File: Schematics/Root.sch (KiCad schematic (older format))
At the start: 1 part, among them CON2 BARREL_JACK

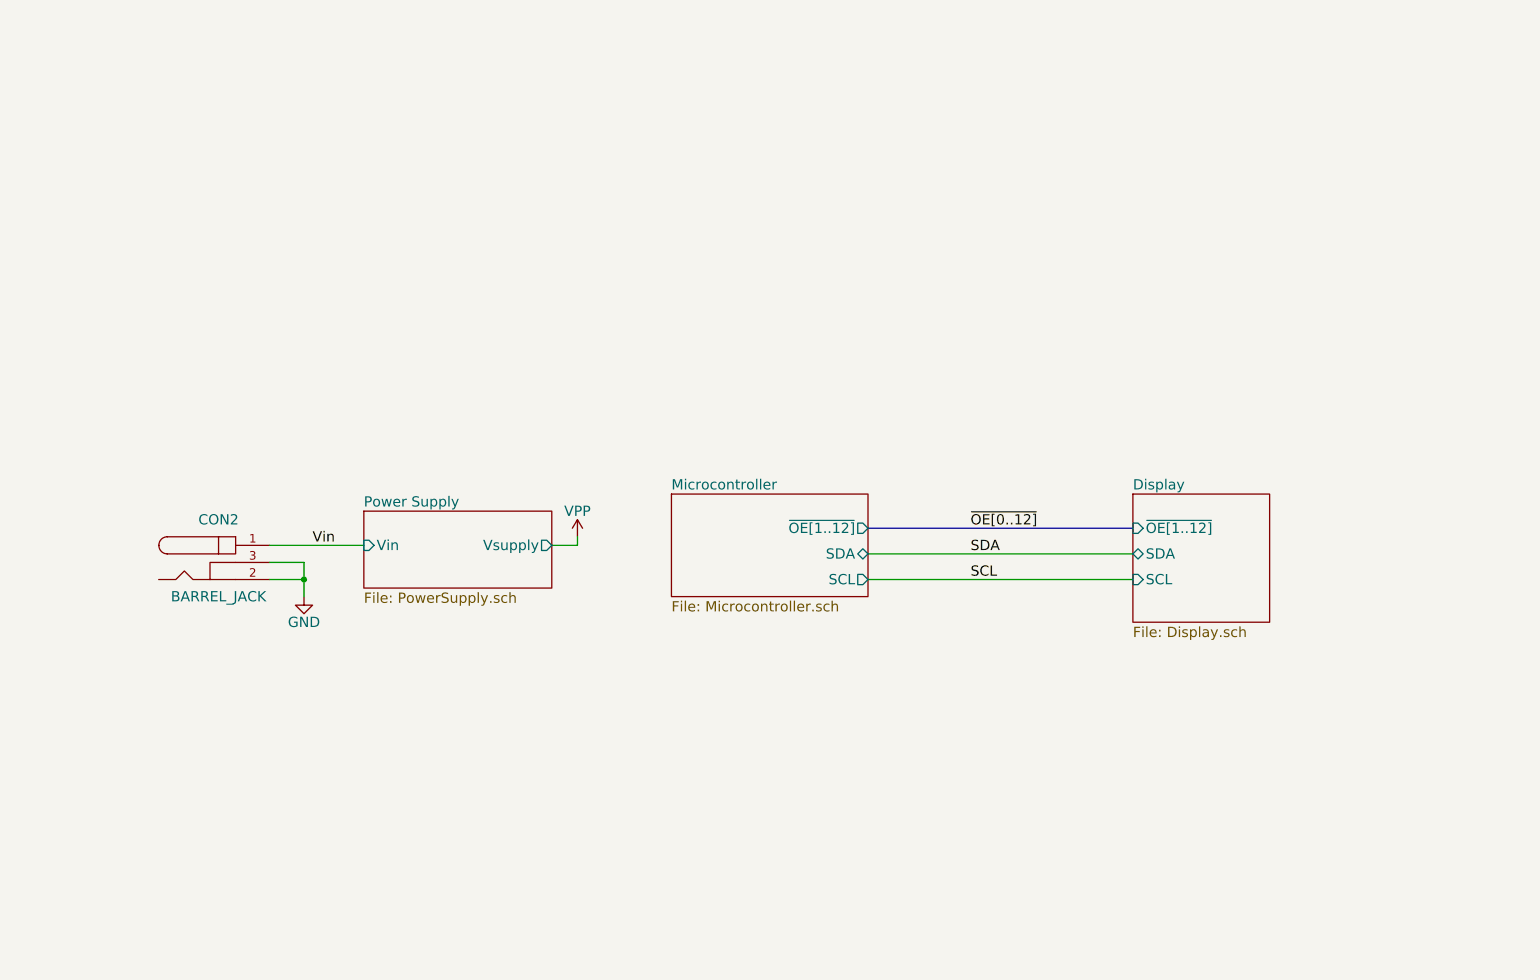
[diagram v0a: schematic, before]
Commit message: Started Redesign.
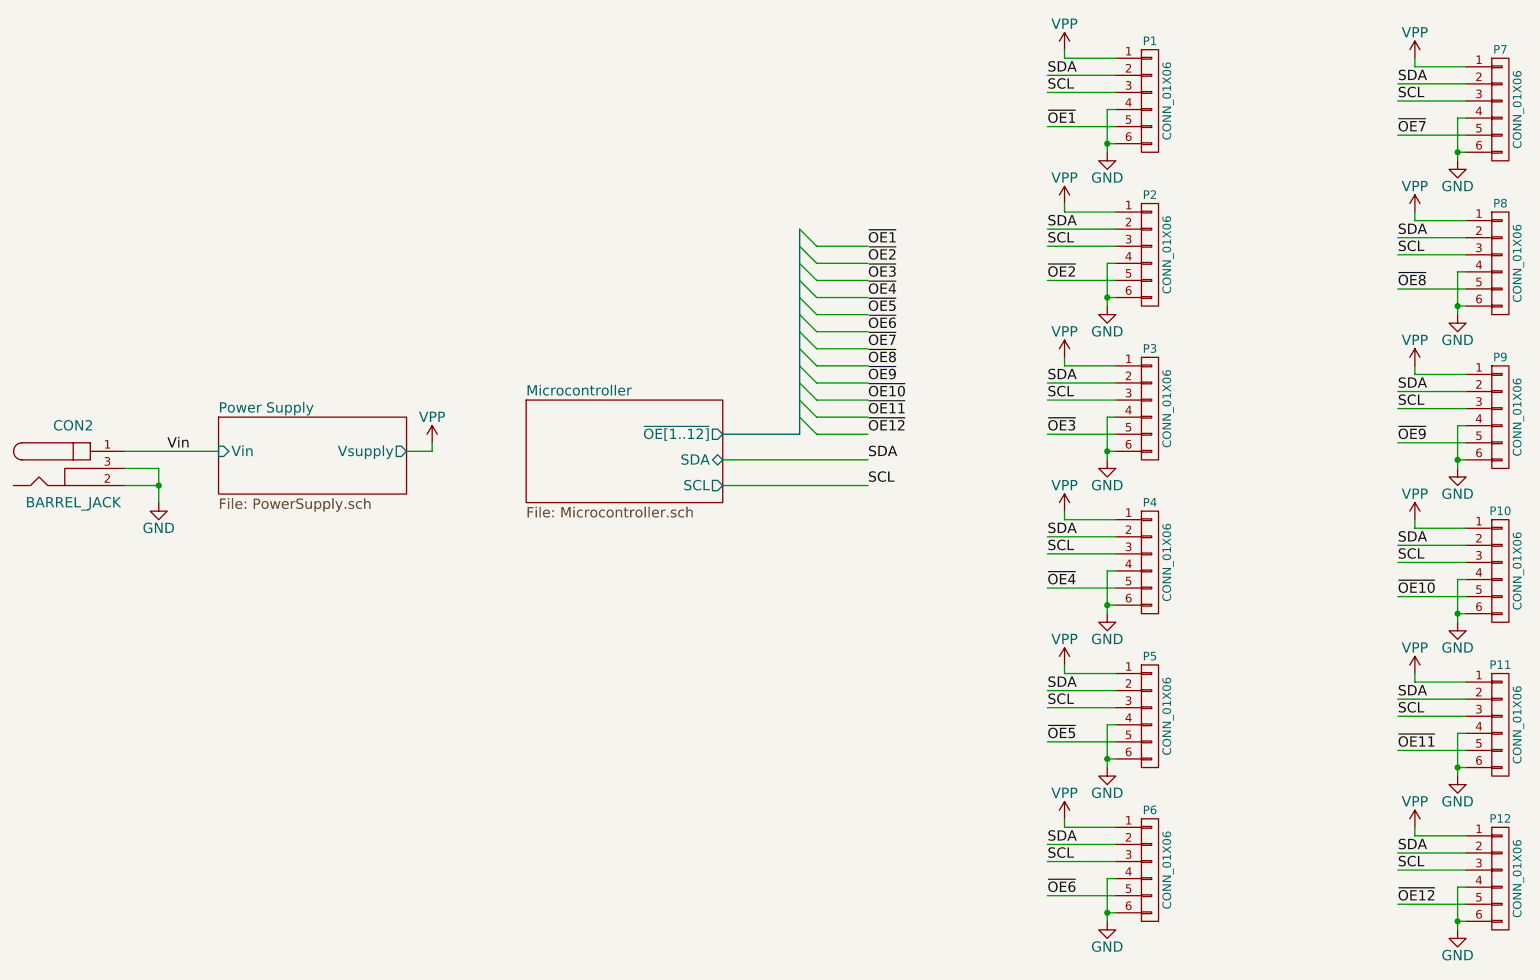
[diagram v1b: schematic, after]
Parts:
- added P1, P10, P11, P12, P2, P3, P4, P5, P6, P7, P8, P9: CONN_01X06, symbol CONN_01X06
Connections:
- net GND: now also P1.4 (P4), P1.6 (P6), P10.4 (P4), P10.6 (P6), P11.4 (P4), P11.6 (P6), P12.4 (P4), P12.6 (P6), P2.4 (P4), P2.6 (P6), P3.4 (P4), P3.6 (P6), P4.4 (P4), P4.6 (P6), P5.4 (P4), P5.6 (P6), P6.4 (P4), P6.6 (P6), P7.4 (P4), P7.6 (P6), P8.4 (P4), P8.6 (P6), P9.4 (P4), P9.6 (P6)
- net SCL: now also P1.3 (P3), P10.3 (P3), P11.3 (P3), P12.3 (P3), P2.3 (P3), P3.3 (P3), P4.3 (P3), P5.3 (P3), P6.3 (P3), P7.3 (P3), P8.3 (P3), P9.3 (P3)
- net SDA: now also P1.2 (P2), P10.2 (P2), P11.2 (P2), P12.2 (P2), P2.2 (P2), P3.2 (P2), P4.2 (P2), P5.2 (P2), P6.2 (P2), P7.2 (P2), P8.2 (P2), P9.2 (P2)
- net VPP: now also P1.1 (P1), P10.1 (P1), P11.1 (P1), P12.1 (P1), P2.1 (P1), P3.1 (P1), P4.1 (P1), P5.1 (P1), P6.1 (P1), P7.1 (P1), P8.1 (P1), P9.1 (P1)
- new net ~OE1: P1.5 (P5)
- new net ~OE10: P10.5 (P5)
- new net ~OE11: P11.5 (P5)
- new net ~OE12: P12.5 (P5)
- new net ~OE2: P2.5 (P5)
- new net ~OE3: P3.5 (P5)
- new net ~OE4: P4.5 (P5)
- new net ~OE5: P5.5 (P5)
- new net ~OE6: P6.5 (P5)
- new net ~OE7: P7.5 (P5)
- new net ~OE8: P8.5 (P5)
- new net ~OE9: P9.5 (P5)
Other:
- moved on the sheet: CON2
